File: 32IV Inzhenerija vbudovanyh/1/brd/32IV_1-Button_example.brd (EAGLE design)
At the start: 91.8 x 85.2 mm, 13 parts, among them U1 ARDUINO-UNO-R3-SHIELD

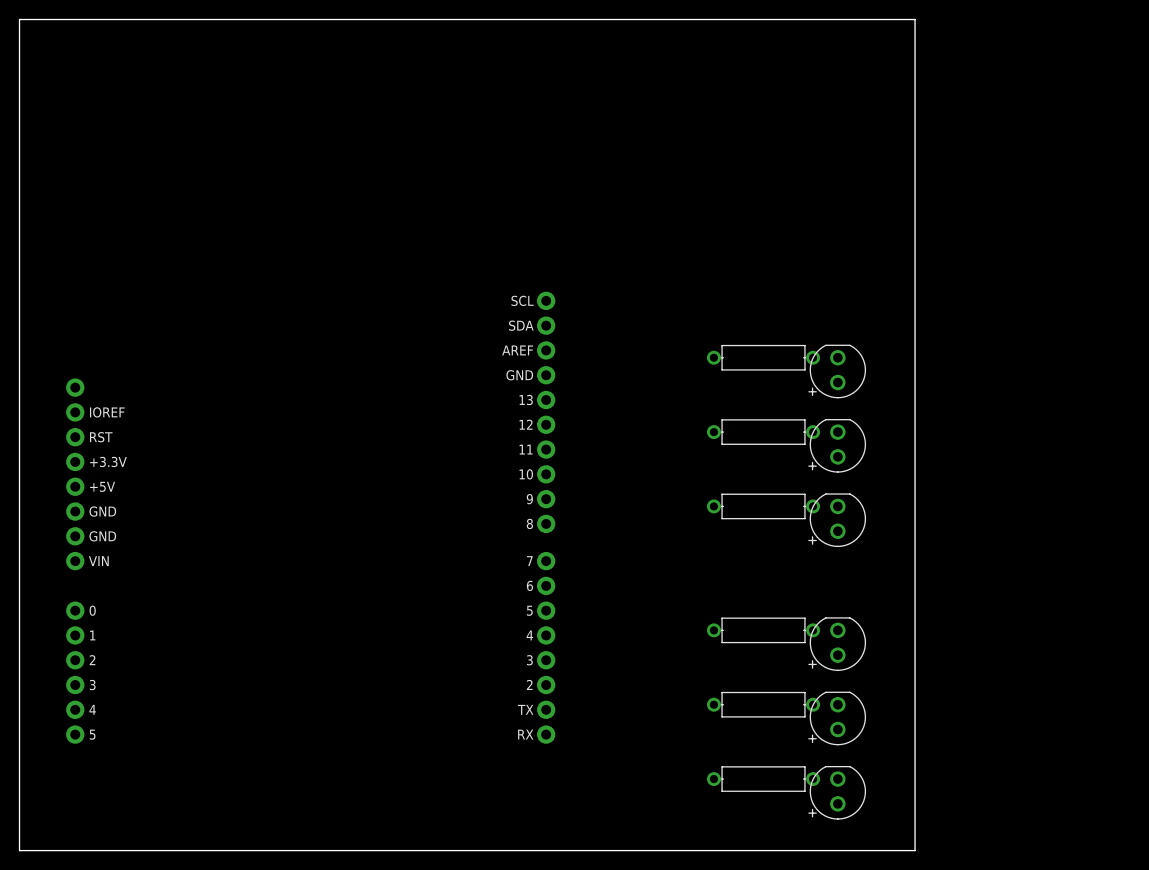
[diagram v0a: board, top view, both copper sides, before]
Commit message: Click to see changes
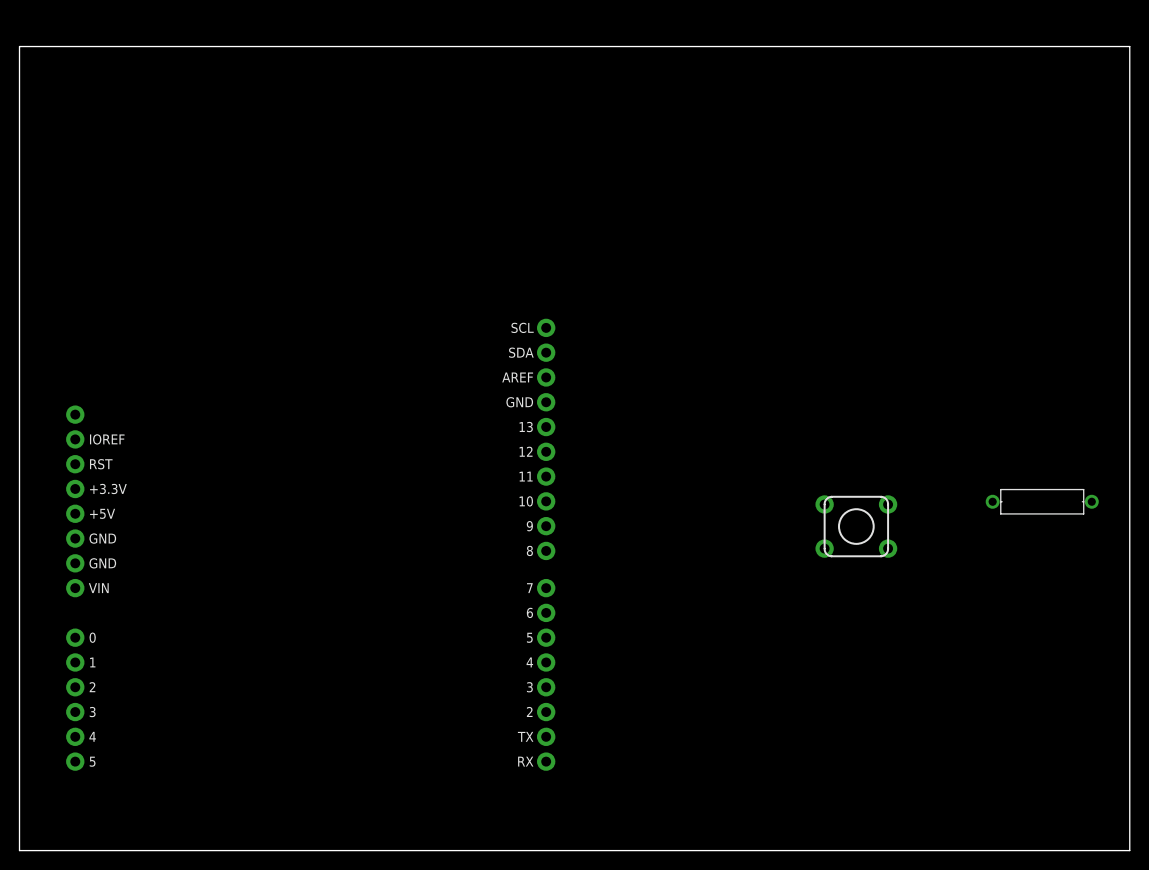
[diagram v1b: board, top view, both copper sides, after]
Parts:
- removed D1, D2, D3, D4, D5, D6: RED, Tinkercad:LEDRD254W60D565H860B
- removed R2, R3, R4, R5, R6, R7: 1k, Tinkercad:RESAD1016W63L850D250B
- added R1: 1k, Tinkercad:RESAD1016W63L850D250B
- added S1: SWITCH_MOMENTARY, Tinkercad:SWITCH-MOMENTARY-PTH-6.5MM
- moved U1 2.77 mm to (29.8, 34.5)
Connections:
- removed net D1_C: D1.2, R2.2
- removed net D2_C: D2.2, R3.2
- removed net D3_C: D3.2, R4.2
- removed net D4_C: D4.2, R5.2
- removed net D5_C: D5.2, R6.2
- removed net D6_C: D6.2, R7.2
- removed net U1_D2: D6.1, U1.D2
- removed net U1_D3: D5.1, U1.D3
- removed net U1_D4: D4.1, U1.D4
- removed net U1_D5: D3.1, U1.D5
- removed net U1_D6: D2.1, U1.D6
- removed net U1_D7: D1.1, U1.D7
- new net U1_5V: S1.3, S1.4, U1.5V
- new net U1_D10: R1.1, S1.1, S1.2, U1.D10
- net U1_GND: now also R1.2; no longer R2.1, R3.1, R4.1, R5.1, R6.1, R7.1
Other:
- board size 91.8 x 85.2 mm -> 113.8 x 82.4 mm
